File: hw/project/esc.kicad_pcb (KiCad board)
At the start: 4 copper layers, 183 parts, among them J1 Battery, J10 I2C, J11 Voltage Monitor, J12 Misc, J2 Phases, J3 FTSH-107-01-L-DV-K-A, J4 Throttle, J5 Hall, J6 Serial, J7 SPI, J8 2.54 Comm, J9 CAN, Q1 SQM50061EL_GE3, Q2 SQM50061EL_GE3, Q3 STL110N10F7, Q4 STL110N10F7, Q5 STL110N10F7, Q6 STL110N10F7, Q7 STL110N10F7, Q8 STL110N10F7, SW1 BOOT0, SW2 RESET, SW3 USER, U1 STSPIN32G4, U2 LMR51610XDBVR, U3 ATA6561-GAQW-N, X1 32MHZ 10PF

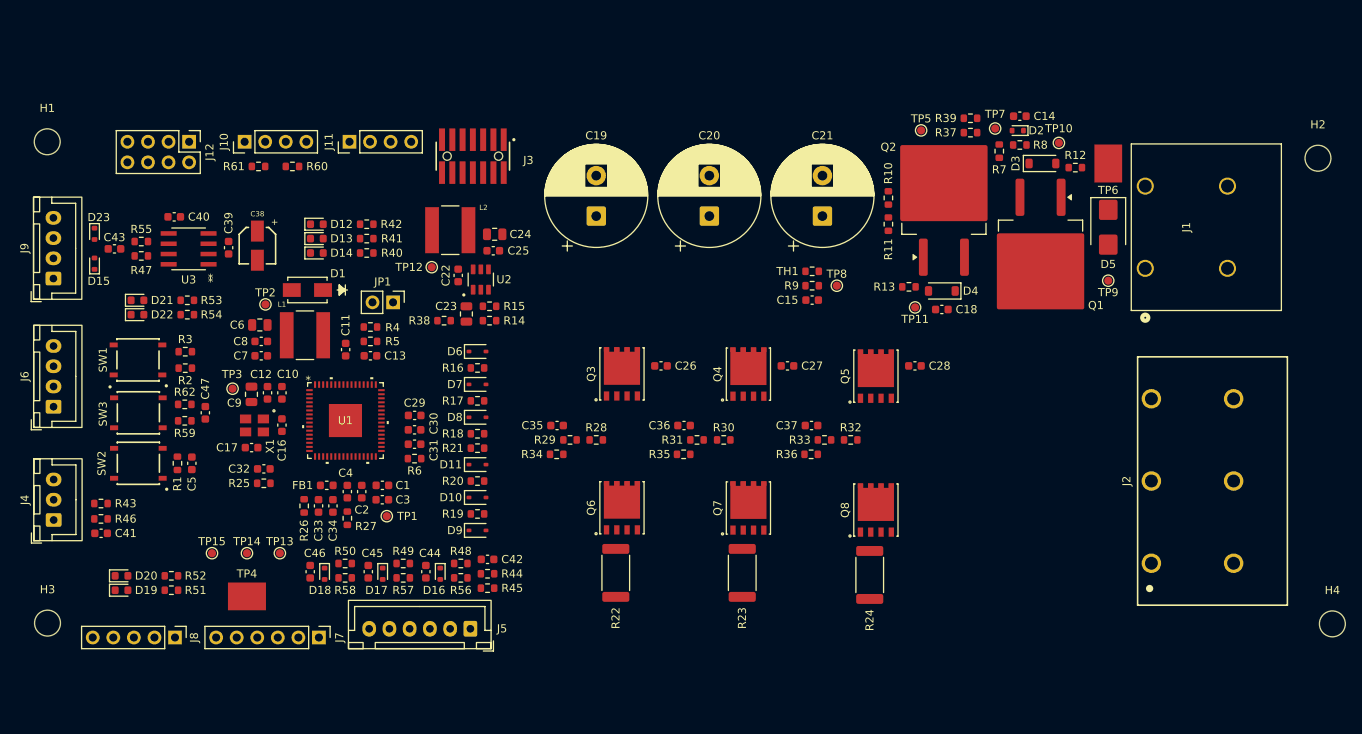
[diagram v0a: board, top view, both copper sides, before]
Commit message: Rotate some parts in drive section
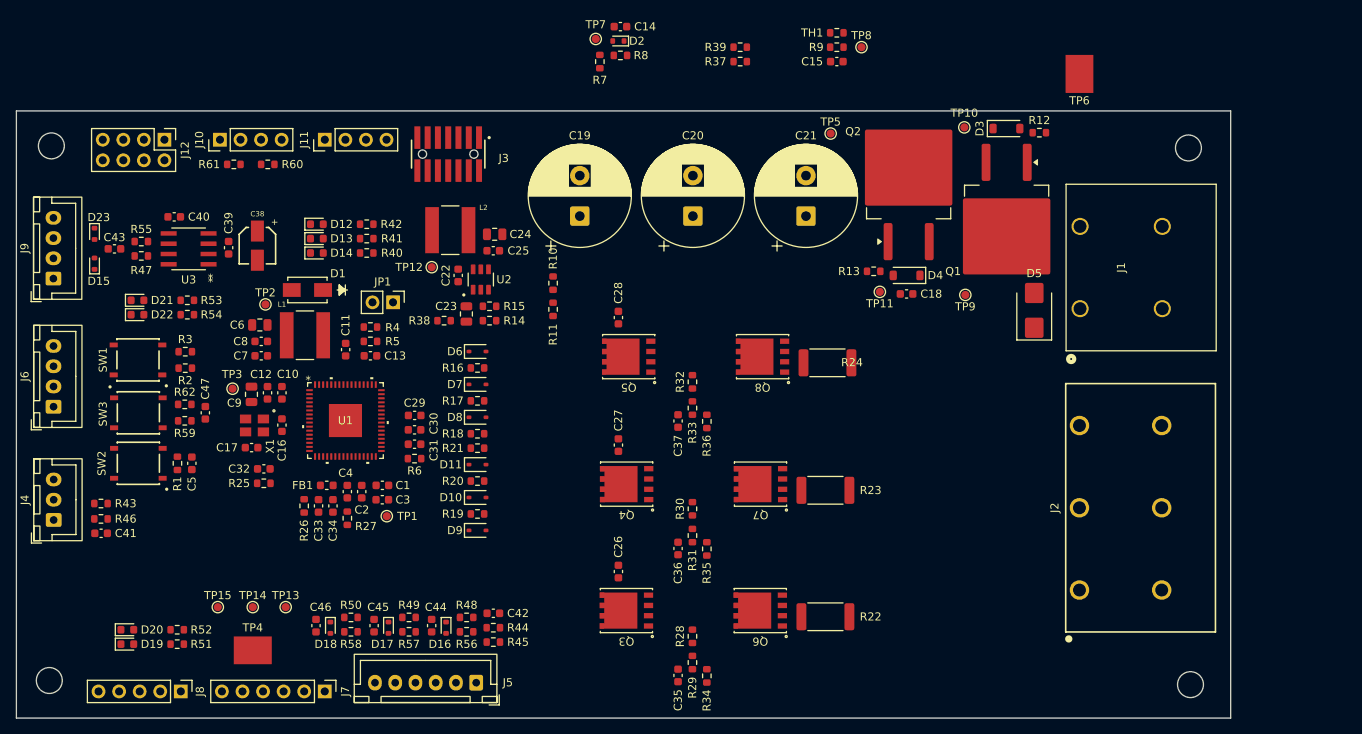
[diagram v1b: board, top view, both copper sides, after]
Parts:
- moved TP7 50.6 mm to (83.5, 3.05)
- moved D2 50.6 mm to (86.3, 3.30)
- moved R7 50.6 mm to (84.0, 5.84)
- moved C14 50.6 mm to (86.6, 1.52)
- moved R8 50.6 mm to (86.6, 5.08)
- moved R10 42.7 mm to (78.2, 33.2)
- moved R11 42.7 mm to (78.2, 36.5)
- moved C28 37.1 mm to (86.3, 37.5), turned to -90 degrees
- moved C35 34.3 mm to (93.7, 81.7), turned to -90 degrees
- moved R34 33.1 mm to (97.2, 81.7), turned to 90 degrees
- moved R29 31.4 mm to (95.4, 80.1), turned to -90 degrees
- moved Q5 30.6 mm to (87.6, 42.3), turned to 180 degrees
- moved R37 29.8 mm to (101.3, 5.84)
- moved R39 29.8 mm to (101.3, 4.06)
- moved C15 29.6 mm to (113.3, 5.84)
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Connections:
- J1 pad 1: /Peripherals/VM_IN -> PGND
- J1 pad 2: /Peripherals/VM_IN -> PGND
- J1 pad 3: PGND -> /Peripherals/VM_IN
- J1 pad 4: PGND -> /Peripherals/VM_IN
- J2 pad 1: /Drive/U -> /Drive/W
- J2 pad 3: /Drive/W -> /Drive/U
- J2 pad A1: /Drive/U -> /Drive/W
- J2 pad A3: /Drive/W -> /Drive/U
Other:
- board outline added: 150 x 75 mm
